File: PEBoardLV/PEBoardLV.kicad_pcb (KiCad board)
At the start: 4 copper layers, 113.7 x 78.7 mm, 72 parts, among them J1 BSPD Test Jumper, J10 ECU Debug Connector, J11 SWD Header, J12 Extra Pin Header, J13 CAN Header, J14 UART Header, J15 To TSAL, J2 Beam Interlock, J3 To HV Interlocks, J4 To Left Panel, J5 To Right Panel, J6 To Brake Light, J7 To PE HV, J8 BSPD Reset, J9 Main LV Connector, U1 MCP6004, U10 ISO1050, U11 STM32F405, U2 4072, U3 4071, U4 DE1A1B-L2-12V, U5 74HC595, U6 LM555N, U7 SN754410, U8 NCP1117-3.3_TO252, U9 L78S05CV-DG, Y1 8MHz

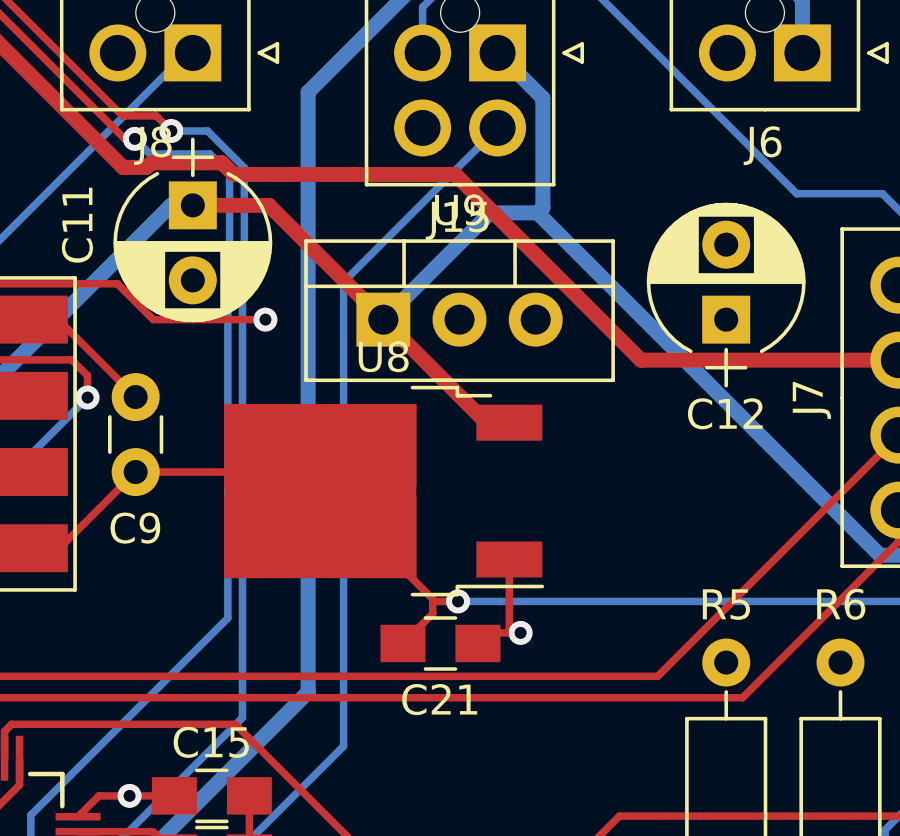
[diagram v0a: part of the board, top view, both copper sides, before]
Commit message: hopefully finalize PCBs for send to manufacturing
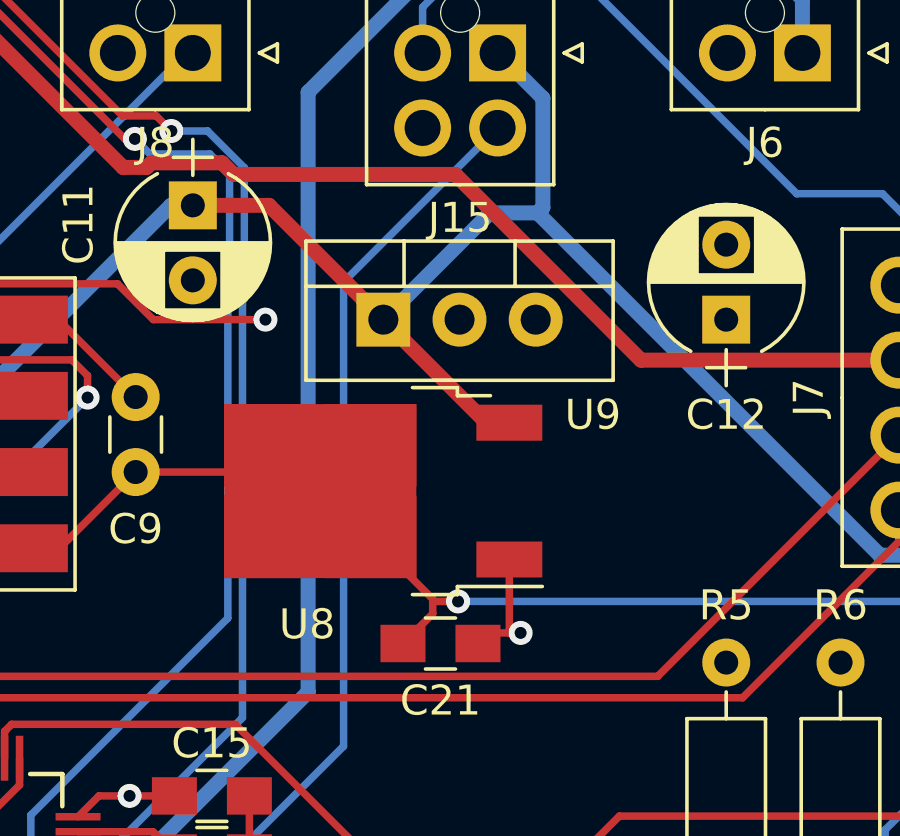
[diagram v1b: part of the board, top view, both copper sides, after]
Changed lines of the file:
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@@
   (layers
     (0 F.Cu signal)
-    (1 In1.Cu power)
+    (1 In1.Cu power hide)
     (2 In2.Cu power hide)
     (31 B.Cu signal)
@@
     (descr "TO-220-3, Vertical, RM 2.54mm")
     (tags "TO-220-3 Vertical RM 2.54mm")
-    (fp_text reference U9 (at 2.54 -3.62) (layer F.SilkS)
+    (fp_text reference U9 (at 6.985 3.175) (layer F.SilkS)
       (effects (font (size 1 1) (thickness 0.15)))
     )
@@
     (tags "DPAK TO-252 DPAK-3 TO-252-3 SOT-428")
     (attr smd)
-    (fp_text reference U8 (at 0 4.445 180) (layer F.SilkS)
+    (fp_text reference U8 (at 2.54 -4.445 180) (layer F.SilkS)
       (effects (font (size 1 1) (thickness 0.15)))
     )
@@
     (effects (font (size 1.5 1.5) (thickness 0.3)))
   )
-  (segment (start 150.495 44.45) (end 152.273 44.45) (width 0.25) (layer In1.Cu) (net 1) (status 400000))
-  (segment (start 159.933 48.3) (end 158.75 48.3) (width 0.25) (layer In1.Cu) (net 1) (status 800000))
+  (segment (start 150.495 44.45) (end 152.273 44.45) (width 0.25) (layer In1.Cu) (net 1))
+  (segment (start 159.933 48.3) (end 158.75 48.3) (width 0.25) (layer In1.Cu) (net 1))
   (segment (start 162.306 50.673) (end 159.933 48.3) (width 0.25) (layer In1.Cu) (net 1))
   (segment (start 162.306 41.148) (end 162.306 50.673) (width 0.25) (layer In1.Cu) (net 1))
@@
   (segment (start 118.4684 52.07) (end 120.44 50.0984) (width 0.25) (layer F.Cu) (net 1))
   (segment (start 118.11 52.07) (end 118.4684 52.07) (width 0.25) (layer F.Cu) (net 1))
-  (segment (start 127 44.45) (end 128.23 44.45) (width 0.25) (layer F.Cu) (net 2) (status C00000))
-  (segment (start 128.23 44.45) (end 130.81 47.03) (width 0.25) (layer F.Cu) (net 2) (status C00000))
+  (segment (start 127 44.45) (end 128.23 44.45) (width 0.25) (layer F.Cu) (net 2))
+  (segment (start 128.23 44.45) (end 130.81 47.03) (width 0.25) (layer F.Cu) (net 2))
   (segment (start 127.0533 44.5033) (end 127 44.45) (width 0.25) (layer F.Cu) (net 2))
   (via (at 125.8938 69.0573) (size 0.8) (layers F.Cu B.Cu) (net 2))
@@
   (segment (start 131.39 61.52) (end 132.1 62.23) (width 0.25) (layer F.Cu) (net 8))
   (segment (start 128.89 61.52) (end 131.39 61.52) (width 0.25) (layer F.Cu) (net 8))
-  (segment (start 127 52.07) (end 128.27 52.07) (width 0.25) (layer F.Cu) (net 9) (status C00000))
-  (segment (start 128.27 52.07) (end 130.81 49.53) (width 0.25) (layer F.Cu) (net 9) (status C00000))
+  (segment (start 127 52.07) (end 128.27 52.07) (width 0.25) (layer F.Cu) (net 9))
+  (segment (start 128.27 52.07) (end 130.81 49.53) (width 0.25) (layer F.Cu) (net 9))
   (via (at 130.6065 60.325) (size 0.8) (layers F.Cu B.Cu) (net 9))
   (via (at 116.86 55.2474) (size 0.8) (layers F.Cu B.Cu) (net 9))
